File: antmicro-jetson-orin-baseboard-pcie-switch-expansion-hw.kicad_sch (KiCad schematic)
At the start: 11 parts, among them J2 Bus_M.2_1-2199230-6

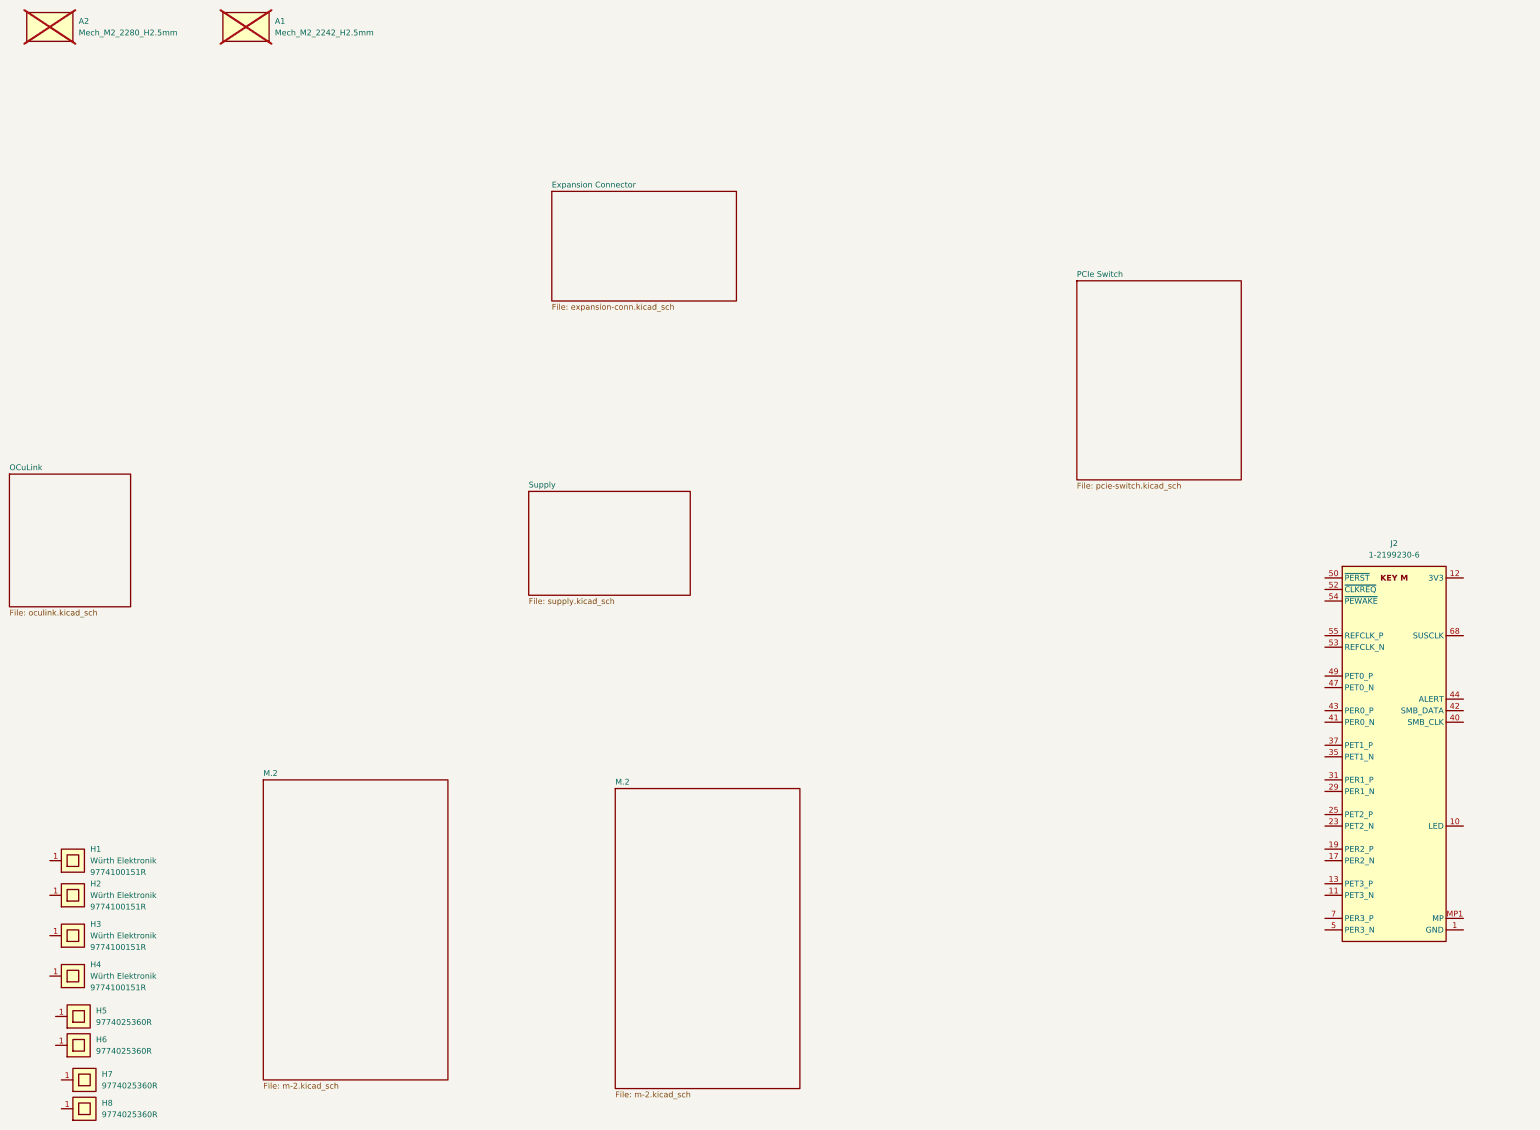
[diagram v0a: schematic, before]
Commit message: [#100765] Update Top Level schematic
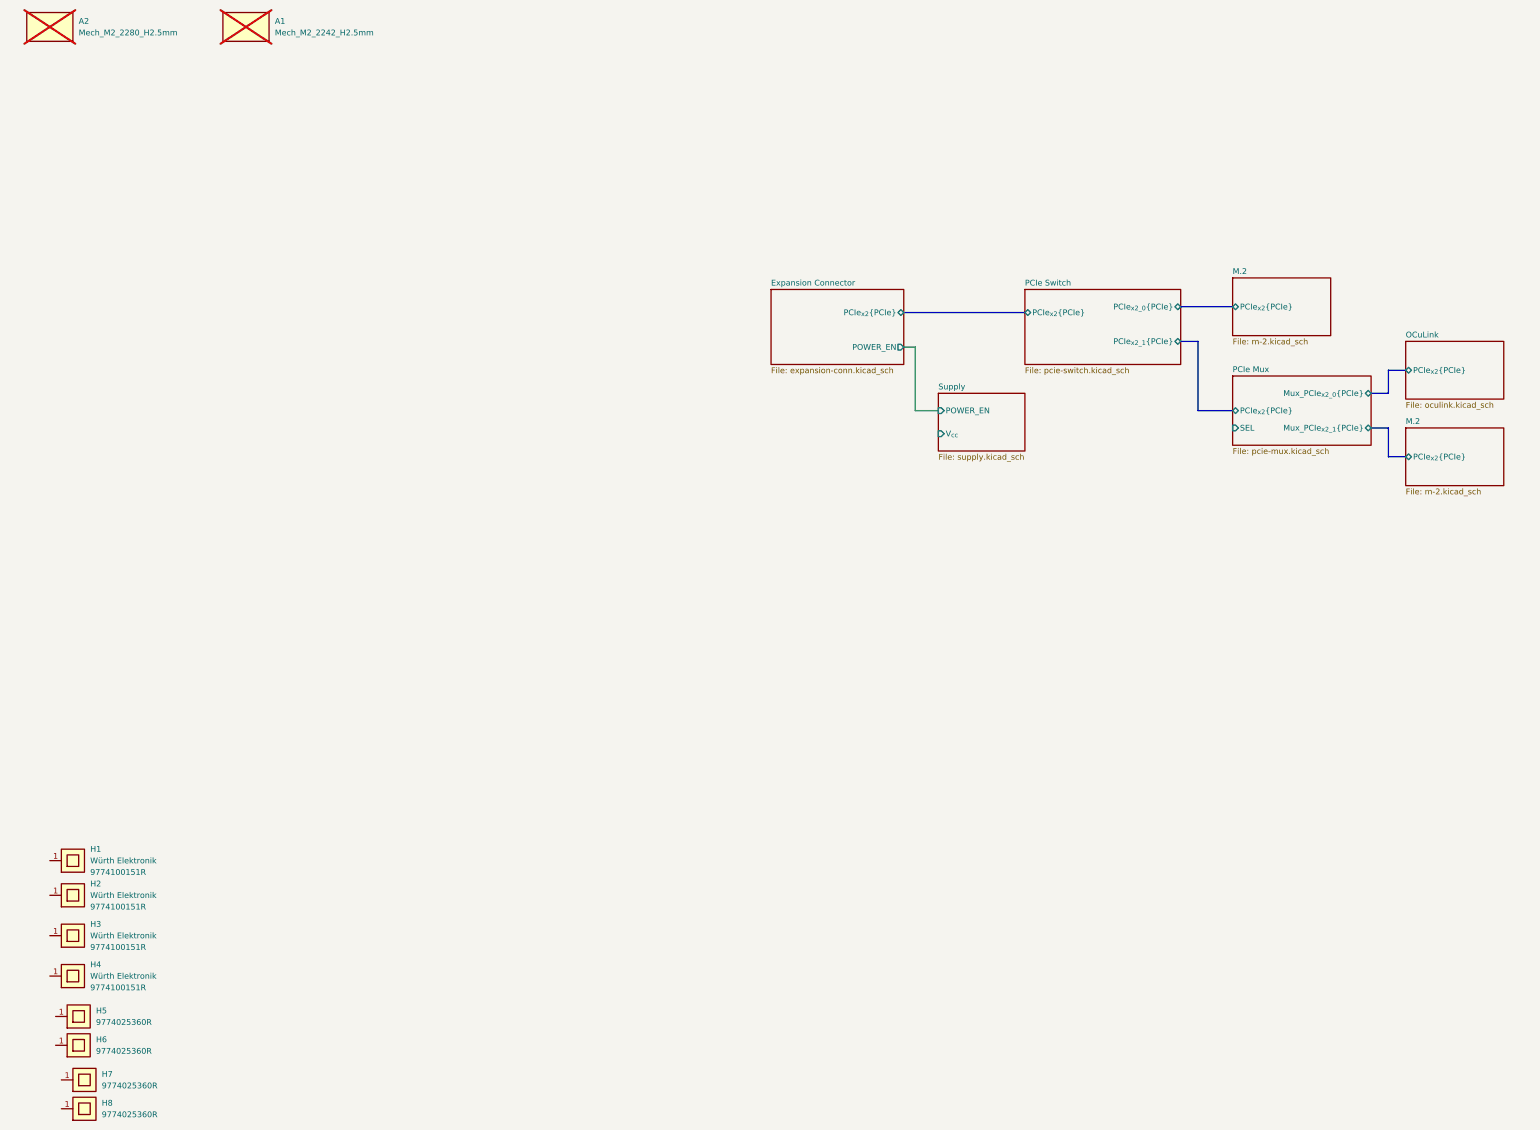
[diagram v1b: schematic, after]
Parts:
- removed J2: Bus_M.2_1-2199230-6, antmicro-footprints:Bus_M.2_Socket_Key_M_TE_1-2199230-6, symbol antmicroPciConnectors:Bus_M.2_1-2199230-6
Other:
- added sheet PCIe Mux (pcie-mux.kicad_sch)
- sheet Expansion Connector ports: added PCIe_{x2}{PCIe}, POWER_EN; removed none
- sheet M.2 ports: added PCIe_{x2}{PCIe}; removed none
- sheet OCuLink ports: added PCIe_{x2}{PCIe}; removed none
- sheet PCIe Switch ports: added PCIe_{x2_0}{PCIe}, PCIe_{x2_1}{PCIe}, PCIe_{x2}{PCIe}; removed none
- sheet Supply ports: added POWER_EN, V_{cc}; removed none
